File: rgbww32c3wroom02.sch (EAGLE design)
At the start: 21 parts, among them IC2 7805TV

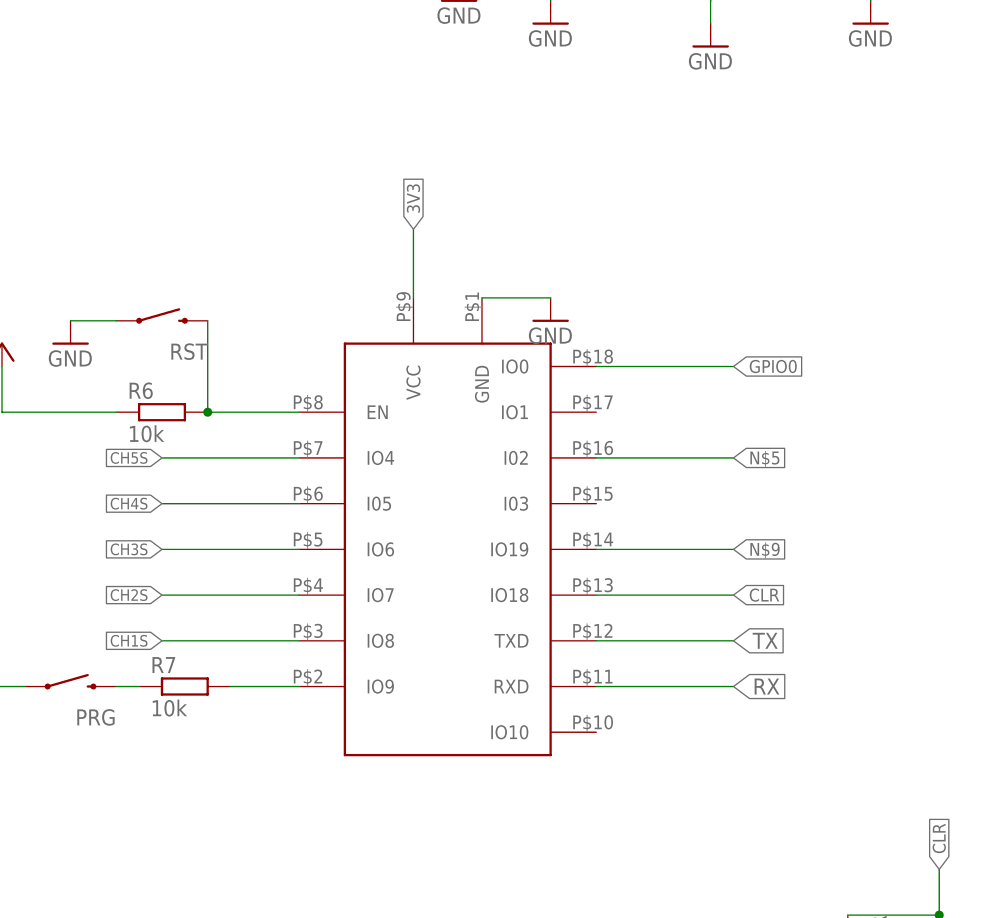
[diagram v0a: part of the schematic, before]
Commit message: some corrections before production
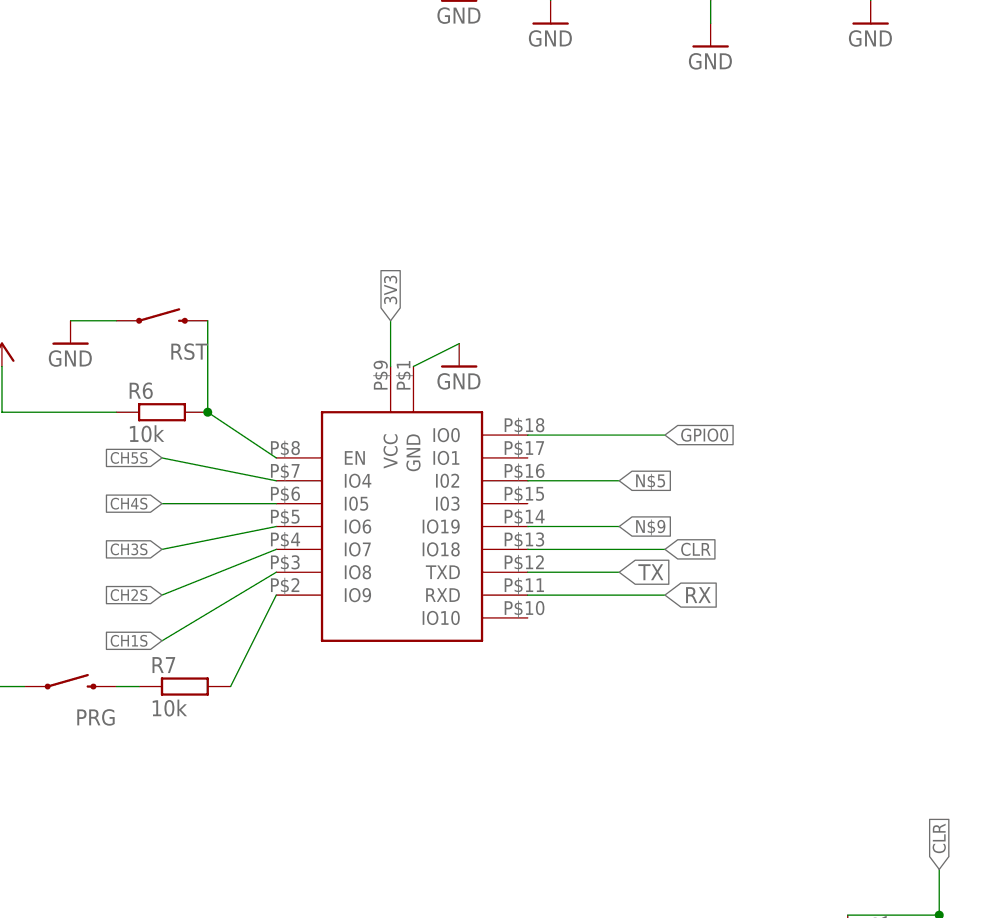
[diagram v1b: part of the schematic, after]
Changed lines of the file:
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@@
 <instance part="R10" gate="G$1" x="-2.54" y="7.62" rot="R90"/>
 <instance part="GND1" gate="1" x="-55.88" y="114.3"/>
-<instance part="GND3" gate="1" x="-45.72" y="78.74"/>
+<instance part="GND3" gate="1" x="-55.88" y="73.66"/>
 <instance part="RST" gate="G$1" x="-88.9" y="78.74" smashed="yes">
 <attribute name="NAME" x="-83.82" y="76.2" size="1.778" layer="95" rot="R180"/>
@@
 <attribute name="VALUE" x="-101.6" y="35.56" size="1.778" layer="96"/>
 </instance>
-<instance part="U$5" gate="G$1" x="-63.5" y="63.5"/>
+<instance part="U$5" gate="G$1" x="-58.42" y="53.34"/>
 </instances>
 <busses>
@@
 </segment>
 <segment>
-<wire x1="-53.34" y1="81.28" x2="-45.72" y2="81.28" width="0.1524" layer="91"/>
+<wire x1="-60.96" y1="73.66" x2="-55.88" y2="76.2" width="0.1524" layer="91"/>
 <pinref part="GND3" gate="1" pin="GND"/>
 <pinref part="U$5" gate="G$1" pin="GND"/>
@@
 <net name="CLR" class="0">
 <segment>
-<wire x1="-40.64" y1="48.26" x2="-25.4" y2="48.26" width="0.1524" layer="91"/>
-<label x="-25.4" y="48.26" size="1.4224" layer="95" xref="yes"/>
+<wire x1="-48.26" y1="53.34" x2="-33.02" y2="53.34" width="0.1524" layer="91"/>
+<label x="-33.02" y="53.34" size="1.4224" layer="95" xref="yes"/>
 <pinref part="U$5" gate="G$1" pin="IO18"/>
 </segment>
@@
 <net name="N$5" class="0">
 <segment>
-<wire x1="-40.64" y1="63.5" x2="-25.4" y2="63.5" width="0.1524" layer="91"/>
-<label x="-25.4" y="63.5" size="1.4224" layer="95" xref="yes"/>
+<wire x1="-48.26" y1="60.96" x2="-38.1" y2="60.96" width="0.1524" layer="91"/>
+<label x="-38.1" y="60.96" size="1.4224" layer="95" xref="yes"/>
 <pinref part="U$5" gate="G$1" pin="I02"/>
 </segment>
@@
 <net name="N$9" class="0">
 <segment>
-<wire x1="-40.64" y1="53.34" x2="-25.4" y2="53.34" width="0.1524" layer="91"/>
-<label x="-25.4" y="53.34" size="1.4224" layer="95" xref="yes"/>
+<wire x1="-48.26" y1="55.88" x2="-38.1" y2="55.88" width="0.1524" layer="91"/>
+<label x="-38.1" y="55.88" size="1.4224" layer="95" xref="yes"/>
 <pinref part="U$5" gate="G$1" pin="IO19"/>
 </segment>
@@
 </segment>
 <segment>
-<wire x1="-60.96" y1="81.28" x2="-60.96" y2="88.9" width="0.1524" layer="91"/>
-<label x="-60.96" y="88.9" size="1.4224" layer="95" rot="R90" xref="yes"/>
+<wire x1="-63.5" y1="73.66" x2="-63.5" y2="78.74" width="0.1524" layer="91"/>
+<label x="-63.5" y="78.74" size="1.4224" layer="95" rot="R90" xref="yes"/>
 <pinref part="U$5" gate="G$1" pin="VCC"/>
 </segment>
@@
 <wire x1="-83.82" y1="78.74" x2="-83.82" y2="68.58" width="0.1524" layer="91"/>
 <pinref part="R6" gate="G$1" pin="2"/>
-<wire x1="-83.82" y1="68.58" x2="-73.66" y2="68.58" width="0.1524" layer="91"/>
+<wire x1="-83.82" y1="68.58" x2="-76.2" y2="63.5" width="0.1524" layer="91"/>
 <junction x="-83.82" y="68.58"/>
 <pinref part="U$5" gate="G$1" pin="EN"/>
@@
 <segment>
 <pinref part="U$5" gate="G$1" pin="IO8"/>
-<wire x1="-73.66" y1="43.18" x2="-88.9" y2="43.18" width="0.1524" layer="91"/>
+<wire x1="-76.2" y1="50.8" x2="-88.9" y2="43.18" width="0.1524" layer="91"/>
 <label x="-88.9" y="43.18" size="1.27" layer="95" rot="R180" xref="yes"/>
 </segment>
@@
 <segment>
 <pinref part="U$5" gate="G$1" pin="IO7"/>
-<wire x1="-73.66" y1="48.26" x2="-88.9" y2="48.26" width="0.1524" layer="91"/>
+<wire x1="-76.2" y1="53.34" x2="-88.9" y2="48.26" width="0.1524" layer="91"/>
 <label x="-88.9" y="48.26" size="1.27" layer="95" rot="R180" xref="yes"/>
 </segment>
@@
 <segment>
 <pinref part="U$5" gate="G$1" pin="IO6"/>
-<wire x1="-73.66" y1="53.34" x2="-88.9" y2="53.34" width="0.1524" layer="91"/>
+<wire x1="-76.2" y1="55.88" x2="-88.9" y2="53.34" width="0.1524" layer="91"/>
 <label x="-88.9" y="53.34" size="1.27" layer="95" rot="R180" xref="yes"/>
 </segment>
@@
 <segment>
 <pinref part="U$5" gate="G$1" pin="I05"/>
-<wire x1="-73.66" y1="58.42" x2="-88.9" y2="58.42" width="0.1524" layer="91"/>
+<wire x1="-76.2" y1="58.42" x2="-88.9" y2="58.42" width="0.1524" layer="91"/>
 <label x="-88.9" y="58.42" size="1.27" layer="95" rot="R180" xref="yes"/>
 </segment>
@@
 <segment>
 <pinref part="U$5" gate="G$1" pin="IO4"/>
-<wire x1="-73.66" y1="63.5" x2="-88.9" y2="63.5" width="0.1524" layer="91"/>
+<wire x1="-76.2" y1="60.96" x2="-88.9" y2="63.5" width="0.1524" layer="91"/>
 <label x="-88.9" y="63.5" size="1.27" layer="95" rot="R180" xref="yes"/>
 </segment>
@@
 </segment>
 <segment>
-<wire x1="-40.64" y1="43.18" x2="-25.4" y2="43.18" width="0.1524" layer="91"/>
-<label x="-25.4" y="43.18" size="1.778" layer="95" xref="yes"/>
+<wire x1="-48.26" y1="50.8" x2="-38.1" y2="50.8" width="0.1524" layer="91"/>
+<label x="-38.1" y="50.8" size="1.778" layer="95" xref="yes"/>
 <pinref part="U$5" gate="G$1" pin="TXD"/>
 </segment>
@@
 </segment>
 <segment>
-<wire x1="-40.64" y1="38.1" x2="-25.4" y2="38.1" width="0.1524" layer="91"/>
-<label x="-25.4" y="38.1" size="1.778" layer="95" xref="yes"/>
+<wire x1="-48.26" y1="48.26" x2="-33.02" y2="48.26" width="0.1524" layer="91"/>
+<label x="-33.02" y="48.26" size="1.778" layer="95" xref="yes"/>
 <pinref part="U$5" gate="G$1" pin="RXD"/>
 </segment>
@@
 </segment>
 <segment>
-<wire x1="-40.64" y1="73.66" x2="-25.4" y2="73.66" width="0.1524" layer="91"/>
-<label x="-25.4" y="73.66" size="1.4224" layer="95" xref="yes"/>
+<wire x1="-48.26" y1="66.04" x2="-33.02" y2="66.04" width="0.1524" layer="91"/>
+<label x="-33.02" y="66.04" size="1.4224" layer="95" xref="yes"/>
 <pinref part="U$5" gate="G$1" pin="IO0"/>
 </segment>
@@
 <segment>
 <pinref part="R7" gate="G$1" pin="2"/>
-<wire x1="-81.28" y1="38.1" x2="-73.66" y2="38.1" width="0.1524" layer="91"/>
+<wire x1="-81.28" y1="38.1" x2="-76.2" y2="48.26" width="0.1524" layer="91"/>
 <pinref part="U$5" gate="G$1" pin="IO9"/>
 </segment>
